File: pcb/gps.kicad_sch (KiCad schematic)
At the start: 2 parts, among them U3 MAX-M10S

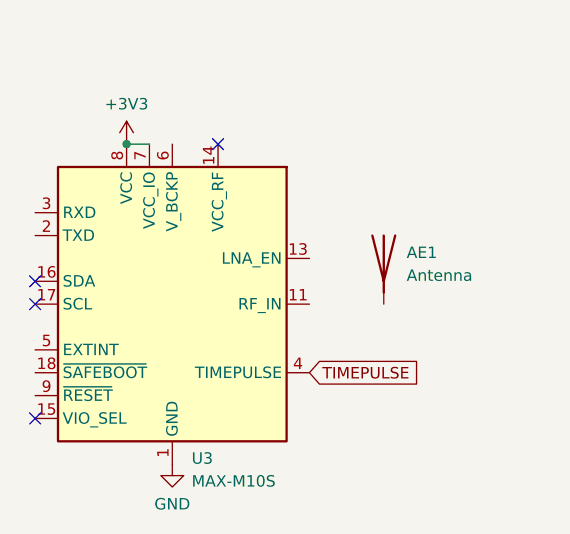
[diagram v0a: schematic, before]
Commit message: sussy
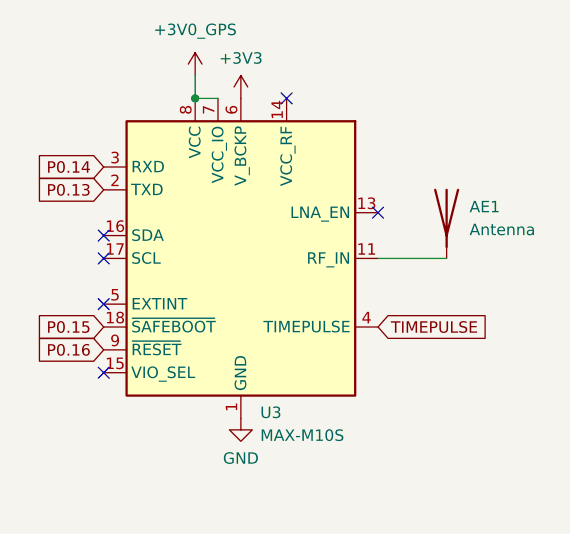
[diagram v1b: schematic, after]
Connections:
- net +3V3: now also U3.6 (V_BCKP); no longer U3.7 (VCC_IO), U3.8 (VCC)
- net at AE1.1 (A): now also U3.11 (RF_IN)
- net P0.15: now reaches U3.18 (~{SAFEBOOT})
- net P0.13: now reaches U3.2 (TXD)
- net P0.14: now reaches U3.3 (RXD)
- net P0.16: now reaches U3.9 (~{RESET})
- new net +3V0_GPS: U3.7 (VCC_IO), U3.8 (VCC)
- no-connect marks 4 -> 6
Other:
- moved on the sheet: AE1, U3
